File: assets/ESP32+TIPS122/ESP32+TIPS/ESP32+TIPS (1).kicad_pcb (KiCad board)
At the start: 2 copper layers, 44 parts, among them J1 Conn_01x03_Pin, J2 DB25_Socket, J3 Screw_Terminal_01x02, Q1 TIP122, Q10 TIP122, Q11 TIP122, Q12 TIP122, Q13 TIP122, Q14 TIP122, Q15 TIP122, Q16 TIP122, Q17 TIP122, Q18 TIP122, Q19 TIP122, Q2 TIP122, Q20 TIP122, Q3 TIP122, Q4 TIP122, Q5 TIP122, Q6 TIP122, Q7 TIP122, Q8 TIP122, Q9 TIP122, U2 ESP32-DEVKIT-V1

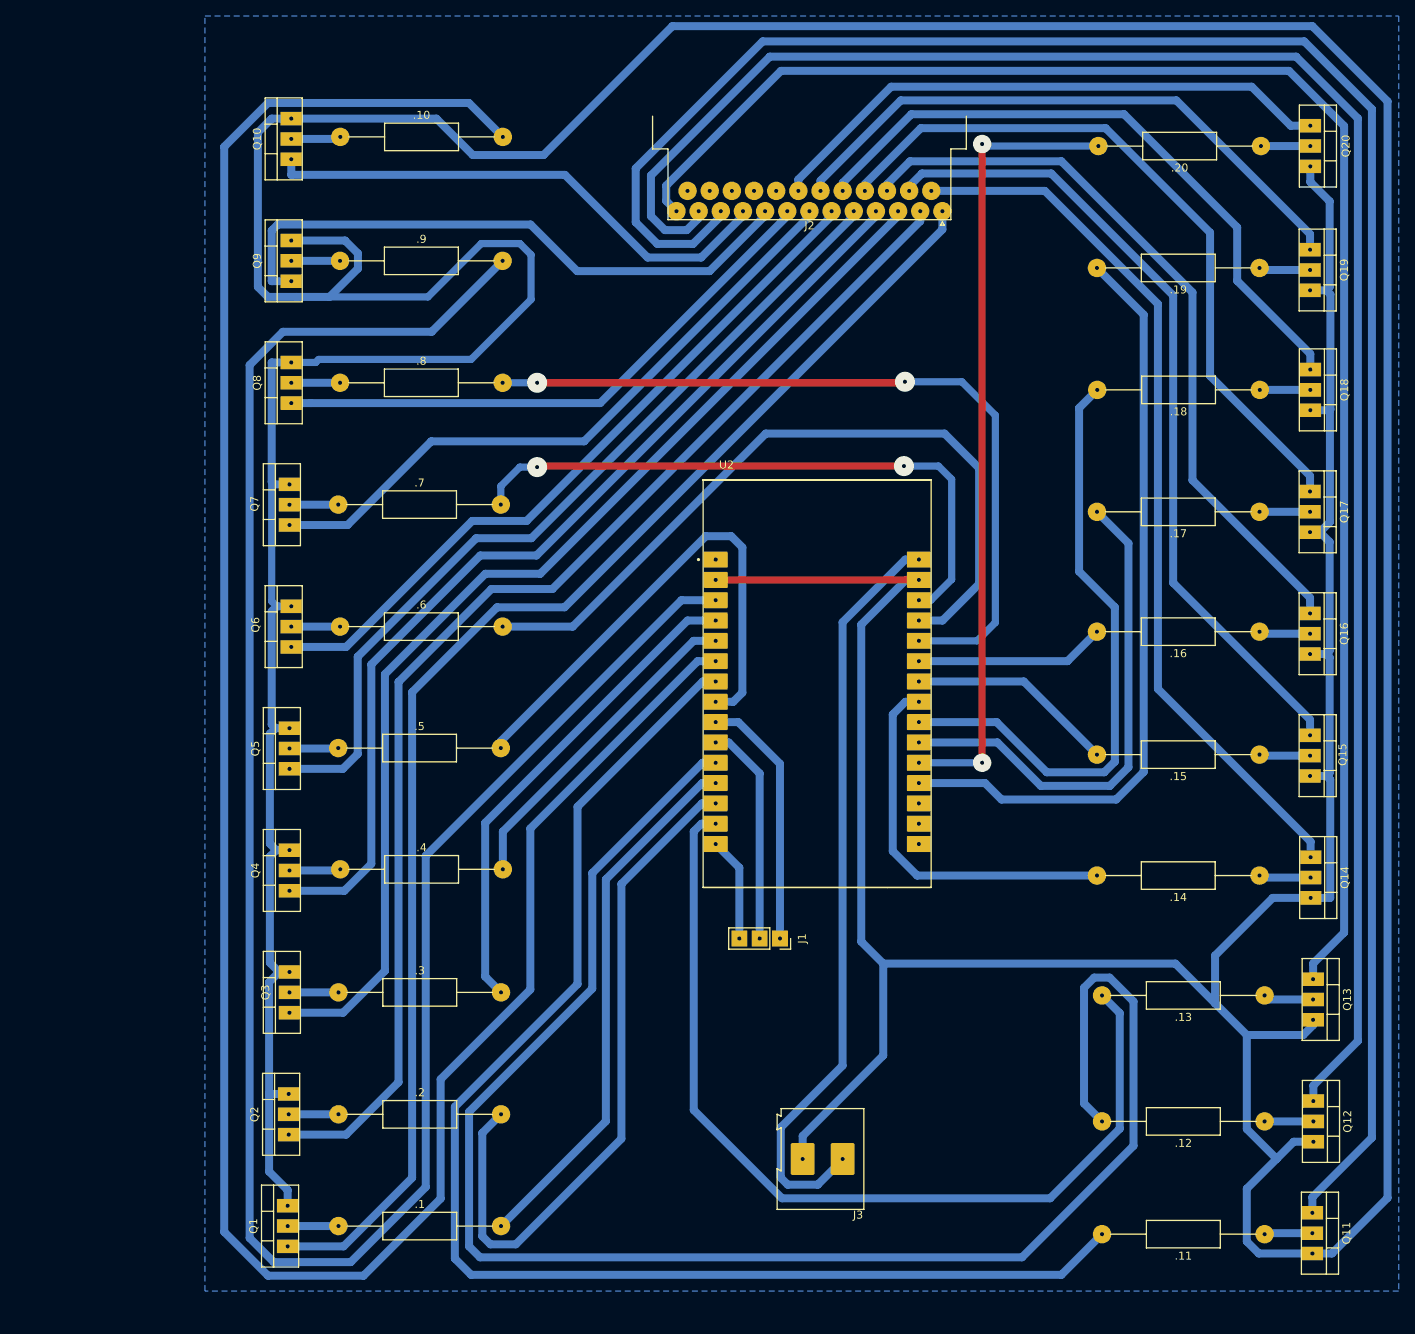
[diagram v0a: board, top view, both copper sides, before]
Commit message: update assets PCB
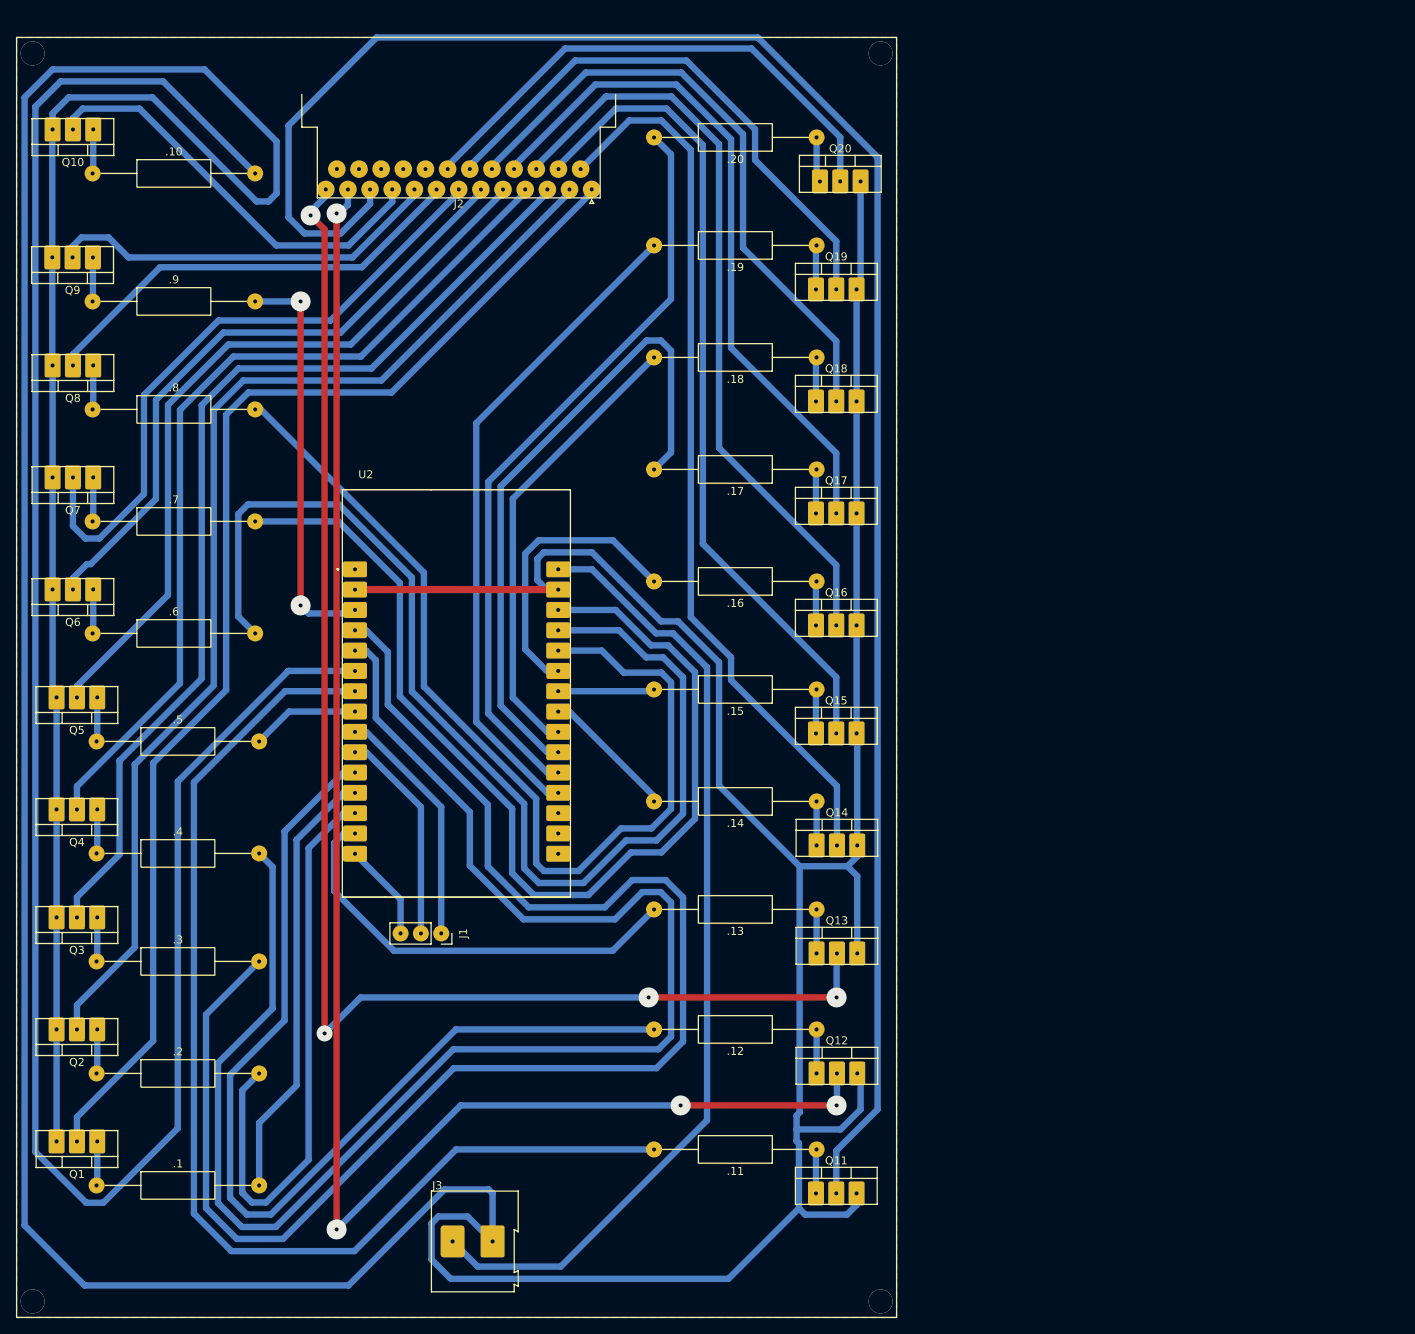
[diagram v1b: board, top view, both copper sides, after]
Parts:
- U2: footprint Battery:MODULE_ESP32_DEVKIT_V1 -> ESP32-DEVKIT-V1:MODULE_ESP32_DEVKIT_V1
- moved Q12 62.2 mm to (142.5, 152.5), turned to 0 degrees
- moved Q13 62.1 mm to (142.5, 137.5), turned to 0 degrees
- moved Q11 62.1 mm to (142.4, 167.5), turned to 0 degrees
- moved Q19 62.0 mm to (142.4, 54.5), turned to 0 degrees
- moved Q18 61.9 mm to (142.4, 68.5), turned to 0 degrees
- moved Q17 61.8 mm to (142.4, 82.5), turned to 0 degrees
- moved Q16 61.8 mm to (142.4, 96.5), turned to 0 degrees
- moved Q14 61.8 mm to (142.5, 124.0), turned to 0 degrees
- moved Q15 61.8 mm to (142.4, 110.0), turned to 0 degrees
- moved Q20 61.7 mm to (142.9, 41.0), turned to 0 degrees
- moved .12 57.2 mm to (142.5, 147.0)
- moved .13 57.0 mm to (142.5, 132.0)
- moved .11 57.0 mm to (142.5, 162.0)
- moved .14 56.1 mm to (142.5, 118.5)
- moved .15 56.0 mm to (142.5, 104.5)
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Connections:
- Q1 pad 1: Net-(Q1-C) -> Net-(Q1-B)
- Q1 pad 2: Net-(Q1-B) -> Net-(Q1-C)
- Q10 pad 1: Net-(Q10-C) -> Net-(Q10-B)
- Q10 pad 2: Net-(Q10-B) -> Net-(Q10-C)
- Q11 pad 1: Net-(Q11-C) -> Net-(Q11-B)
- Q11 pad 2: Net-(Q11-B) -> Net-(Q11-C)
- Q12 pad 1: Net-(Q12-C) -> Net-(Q12-B)
- Q12 pad 2: Net-(Q12-B) -> Net-(Q12-C)
- Q13 pad 1: Net-(Q13-C) -> Net-(Q13-B)
- Q13 pad 2: Net-(Q13-B) -> Net-(Q13-C)
- Q14 pad 1: Net-(J2-P14) -> Net-(Q14-B)
- Q14 pad 2: Net-(Q14-B) -> Net-(J2-P14)
- Q15 pad 1: Net-(J2-P15) -> Net-(Q15-B)
- Q15 pad 2: Net-(Q15-B) -> Net-(J2-P15)
- Q16 pad 1: Net-(J2-P16) -> Net-(Q16-B)
- Q16 pad 2: Net-(Q16-B) -> Net-(J2-P16)
- Q17 pad 1: Net-(J2-P17) -> Net-(Q17-B)
- Q17 pad 2: Net-(Q17-B) -> Net-(J2-P17)
- Q18 pad 1: Net-(J2-P18) -> Net-(Q18-B)
- Q18 pad 2: Net-(Q18-B) -> Net-(J2-P18)
- Q19 pad 1: Net-(J2-P19) -> Net-(Q19-B)
- Q19 pad 2: Net-(Q19-B) -> Net-(J2-P19)
- Q2 pad 1: Net-(Q2-C) -> Net-(Q2-B)
- Q2 pad 2: Net-(Q2-B) -> Net-(Q2-C)
- Q20 pad 1: Net-(J2-P20) -> Net-(Q20-B)
- Q20 pad 2: Net-(Q20-B) -> Net-(J2-P20)
- Q3 pad 1: Net-(Q3-C) -> Net-(Q3-B)
- Q3 pad 2: Net-(Q3-B) -> Net-(Q3-C)
- Q4 pad 1: Net-(Q4-C) -> Net-(Q4-B)
- Q4 pad 2: Net-(Q4-B) -> Net-(Q4-C)
- Q5 pad 1: Net-(Q5-C) -> Net-(Q5-B)
- Q5 pad 2: Net-(Q5-B) -> Net-(Q5-C)
- Q6 pad 1: Net-(Q6-C) -> Net-(Q6-B)
- Q6 pad 2: Net-(Q6-B) -> Net-(Q6-C)
- Q7 pad 1: Net-(Q7-C) -> Net-(Q7-B)
- Q7 pad 2: Net-(Q7-B) -> Net-(Q7-C)
- Q8 pad 1: Net-(Q8-C) -> Net-(Q8-B)
- Q8 pad 2: Net-(Q8-B) -> Net-(Q8-C)
- Q9 pad 1: Net-(Q9-C) -> Net-(Q9-B)
- Q9 pad 2: Net-(Q9-B) -> Net-(Q9-C)
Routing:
- net Net-(U2-D15): track 264.2 -> 51.1 mm, vias 0 -> 2
- net Net-(U2-D4): track 41.2 -> 195.2 mm
- net GND: track 880.5 -> 744.2 mm
- net Net-(U2-D2): track 61.3 -> 189.1 mm
- net Net-(U2-D21): track 207.2 -> 123.9 mm
- net Net-(U2-D22): track 117.0 -> 54.3 mm
- net Net-(U2-D13): track 78.1 -> 130.0 mm, vias 2 -> 0
- net Net-(U2-D5): track 64.2 -> 13.5 mm
- net Net-(U2-D12): track 95.2 -> 143.2 mm
- net Net-(Q12-C): track 236.1 -> 203.7 mm, vias 0 -> 4
- net Net-(U2-RX2): track 290.5 -> 259.7 mm
- net Net-(U2-D25): track 47.8 -> 17.0 mm
- net Net-(Q13-C): track 205.5 -> 178.4 mm, vias 0 -> 4
- net Net-(Q9-C): track 76.6 -> 49.6 mm
- net Net-(U2-TX2): track 170.4 -> 143.5 mm
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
